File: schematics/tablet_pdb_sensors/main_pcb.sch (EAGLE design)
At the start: 10 parts

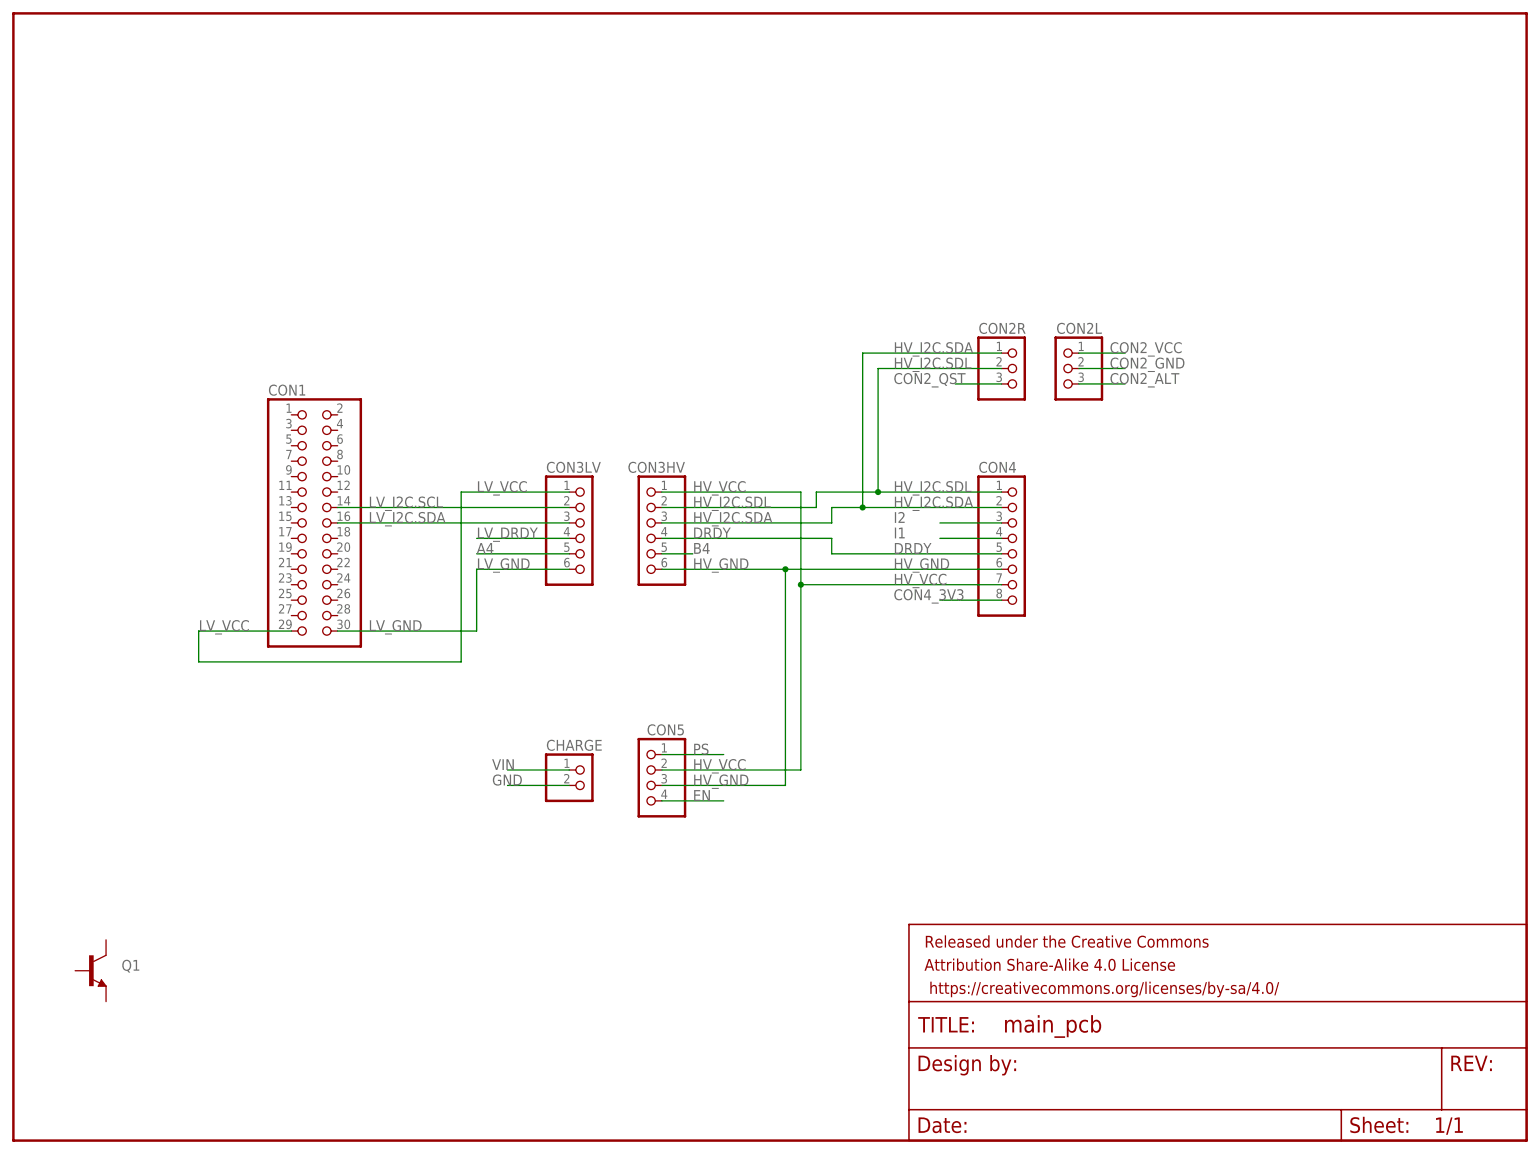
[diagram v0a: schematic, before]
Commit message: Completed schematic
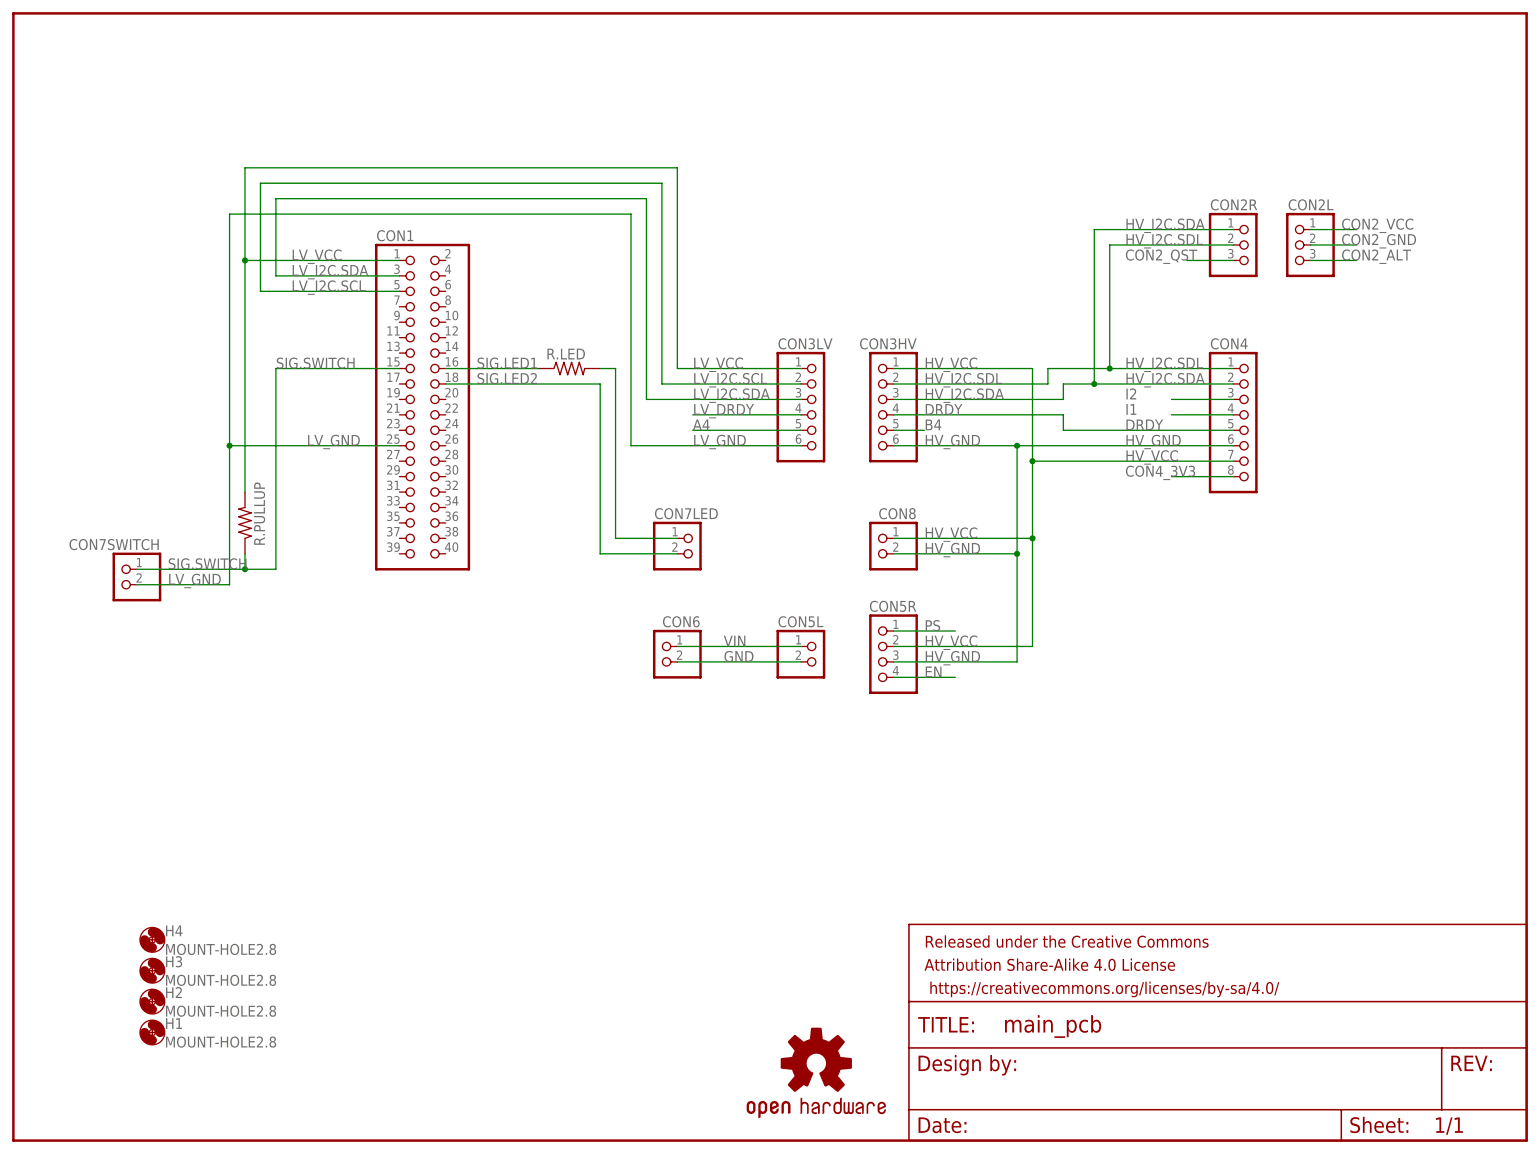
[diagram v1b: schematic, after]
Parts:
- removed CHARGE: (no value), pinhead:PINHD-1X2
- removed CON5: (no value), pinhead:PINHD-1X4
- removed Q1: (no value), SparkFun-DiscreteSemi:TRANSISTOR_NPN2N3904
- added CON5L, CON6, CON7LED, CON7SWITCH, CON8: (no value), pinhead:PINHD-1X2
- added CON5R: (no value), pinhead:PINHD-1X4
- added H1, H2, H3, H4: MOUNT-HOLE2.8, holes:MOUNT-HOLE2.8
- added LOGO1: OSHW-LOGOL, SparkFun-Aesthetics:OSHW-LOGOL
- added R.LED, R.PULLUP: (no value), resistor:R-US_0204/2V
- CON1: device pinhead-2:PINHD-2X15_2.00 -> pinhead:PINHD-2X20
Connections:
- new net N$1: CON7LED.1, R.LED.2
- new net SIG.LED1: CON1.16, R.LED.1
- new net SIG.LED2: CON1.18, CON7LED.2
- new net SIG.SWITCH: CON1.15, CON7SWITCH.1, R.PULLUP.1
- net EN: now also CON5R.4; no longer CON5.4
- net GND: now also CON5L.2, CON6.2; no longer CHARGE.2
- net HV_GND: now also CON5R.3, CON8.2; no longer CON5.3
- net HV_VCC: now also CON5R.2, CON8.1; no longer CON5.2
- net LV_GND: now also CON1.25, CON7SWITCH.2; no longer CON1.30
- net LV_I2C.SCL: now also CON1.5; no longer CON1.14
- net LV_I2C.SDA: now also CON1.3; no longer CON1.16
- net LV_VCC: now also CON1.1, R.PULLUP.2; no longer CON1.29
- net PS: now also CON5R.1; no longer CON5.1
- net VIN: now also CON5L.1, CON6.1; no longer CHARGE.1
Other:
- moved on the sheet: CON2L, CON2R, CON3HV, CON3LV, CON4
